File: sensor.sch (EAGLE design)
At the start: 19 parts

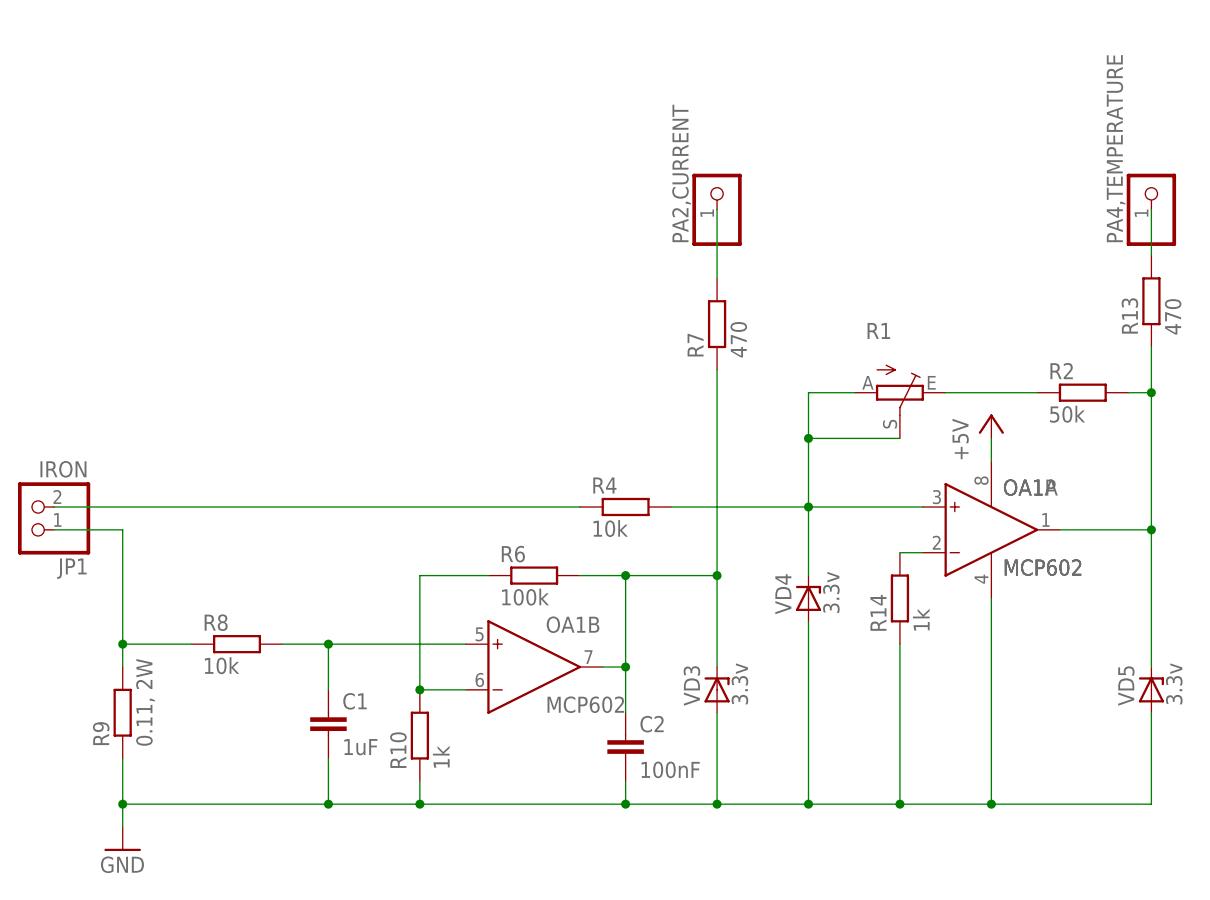
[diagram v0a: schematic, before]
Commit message: Add files via upload
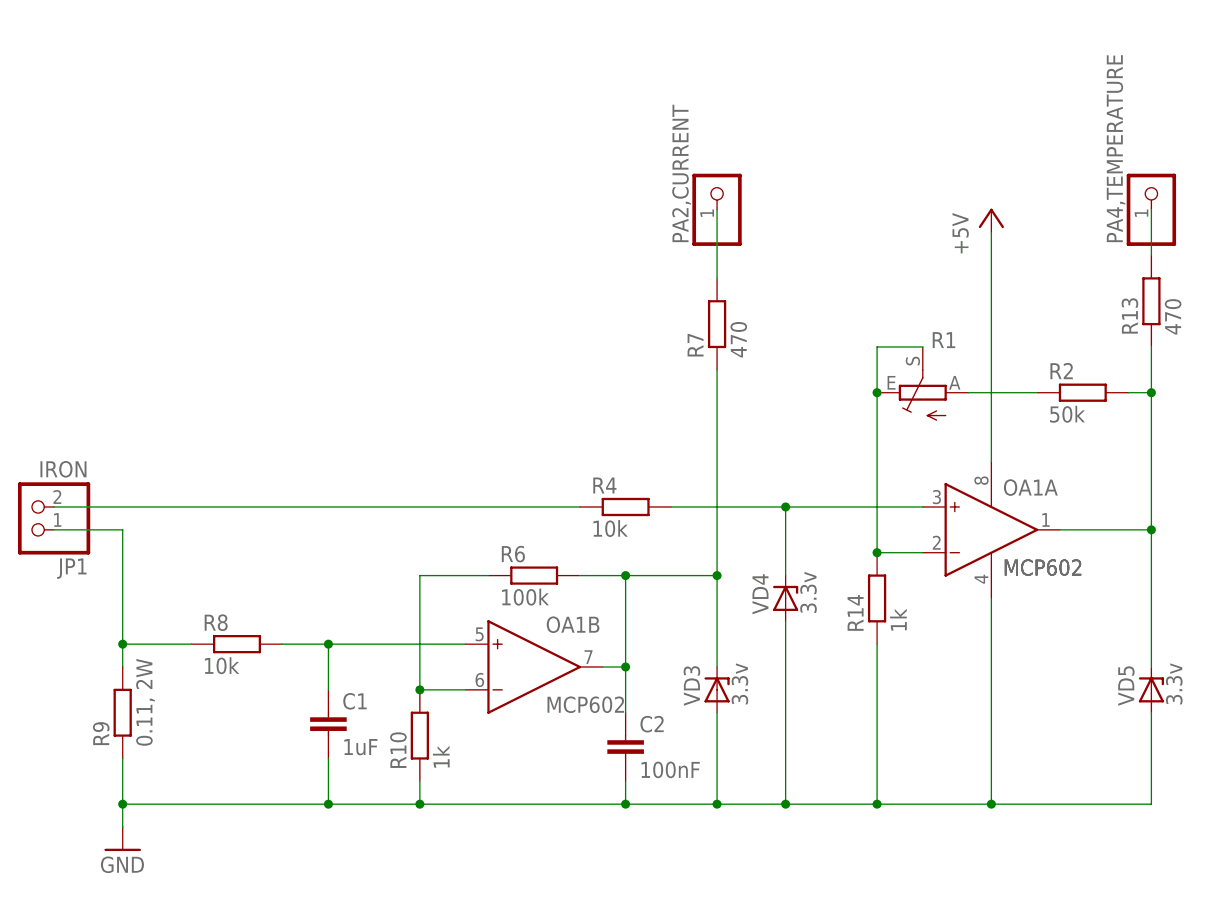
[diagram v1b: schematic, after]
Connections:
- net N$10: now also R1.A; no longer R1.E
- net N$5: no longer R1.A, R1.S
- net N$6: now also R1.E, R1.S
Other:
- moved on the sheet: R1, R14, VD4

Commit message: Add files via upload
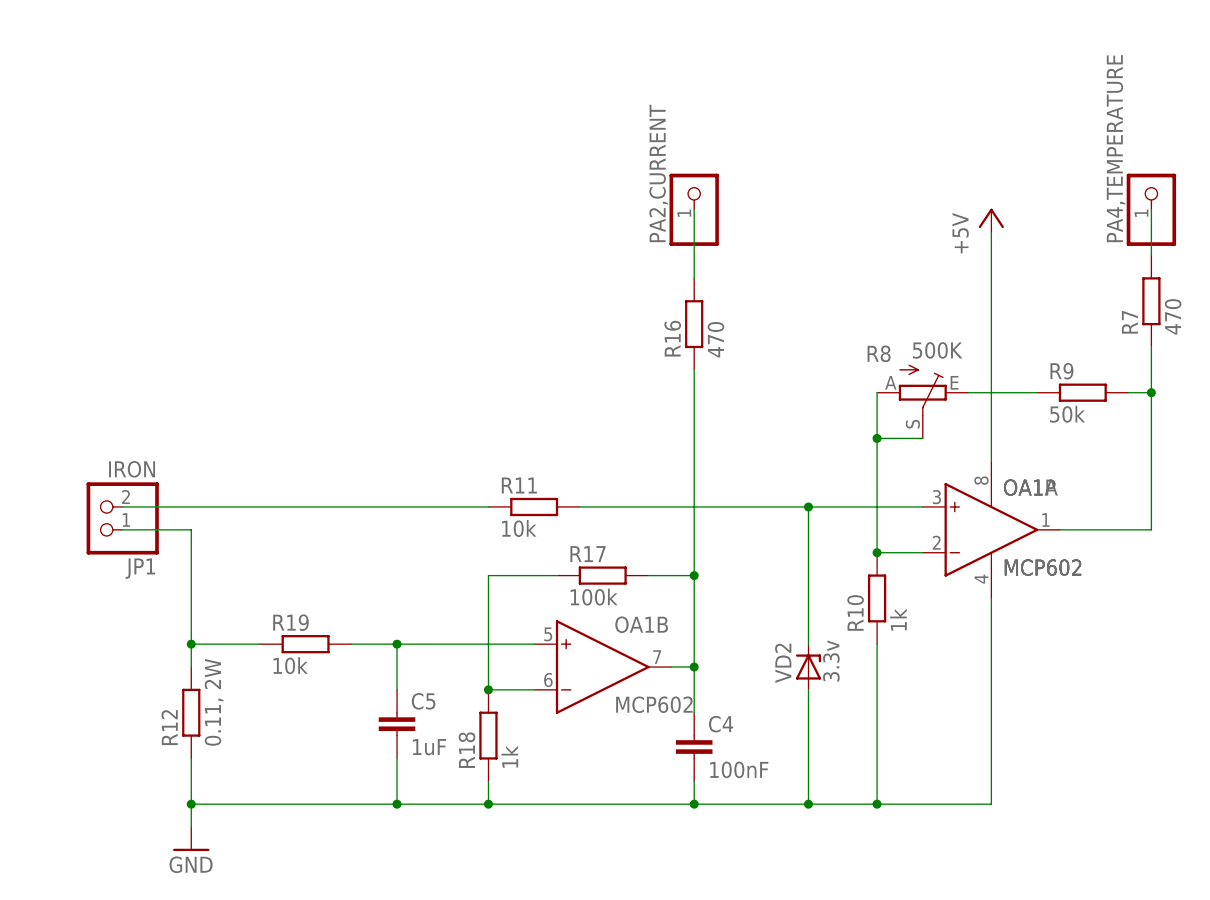
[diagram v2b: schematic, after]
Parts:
- removed C1: 1uF, rcl:C-EU025-024X044
- removed C2: 100nF, rcl:C-EU025-024X044
- removed R1: (no value), pot:TRIM_EU-B64Y
- removed R13: 470, rcl:R-EU_0204/5
- removed R14: 1k, rcl:R-EU_0204/5
- removed R2: 50k, rcl:R-EU_0204/5
- removed R4: 10k, rcl:R-EU_0204/5
- removed R6: 100k, rcl:R-EU_0204/5
- removed VD3, VD4, VD5: 3.3v, diode:ZENER-DIODEC1702-15
- added C4: 100nF, rcl:C-EU025-024X044
- added C5: 1uF, rcl:C-EU025-024X044
- added R11, R19: 10k, rcl:R-EU_0204/5
- added R12: 0.11, 2W, rcl:R-EU_0204/5
- added R16: 470, rcl:R-EU_0204/5
- added R17: 100k, rcl:R-EU_0204/5
- added R18: 1k, rcl:R-EU_0204/5
- added VD2: 3.3v, diode:ZENER-DIODEC1702-15
- R8: value 10k -> 500K; device rcl:R-EU_0204/5 -> pot:TRIM_EU-B64Y
- R9: value 0.11, 2W -> 50k
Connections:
- net GND: now also C4.2, C5.2, R12.1, R18.1, VD2.A; no longer C1.2, C2.2, R14.1, R9.1, VD3.A, VD4.A, VD5.A
- net N$1: now also R12.2, R19.1; no longer R8.1, R9.2
- net N$10: now also R8.E, R9.1; no longer R1.A, R2.1
- net N$11: now also R7.1, R9.2; no longer R13.1, R2.2, VD5.C
- net N$2: now also C5.1, R19.2; no longer C1.1, R8.2
- net N$3: now also R17.1, R18.2; no longer R10.2, R6.1
- net N$4: now also C4.1, R16.1, R17.2; no longer C2.1, R6.2, R7.1, VD3.C
- net N$5: now also R11.2, VD2.C; no longer R4.2, VD4.C
- net N$6: now also R10.2, R8.A, R8.S; no longer R1.E, R1.S, R14.2
- net N$7: now also R11.1; no longer R4.1
- net N$8: now also R16.2; no longer R7.2
- net N$9: now also R7.2; no longer R13.2
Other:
- moved on the sheet: JP1, OA1B, PA2,CURRENT, R10, R7, R9
